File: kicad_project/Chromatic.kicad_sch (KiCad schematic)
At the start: 157 parts

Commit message: arrumadas as bibliotecas
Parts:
- SW_0_R0C0, SW_0_R0C1, SW_0_R0C10, SW_0_R0C11, SW_0_R0C12, SW_0_R0C13, SW_0_R0C14, SW_0_R0C15, SW_0_R0C16, SW_0_R0C2, SW_0_R0C3, SW_0_R0C4, SW_0_R0C5, SW_0_R0C6, SW_0_R0C7, SW_0_R0C8, SW_0_R0C9, SW_1_R1C0, SW_1_R1C1, SW_1_R1C10, SW_1_R1C11, SW_1_R1C12, SW_1_R1C13, SW_1_R1C14, SW_1_R1C15, SW_1_R1C16, SW_1_R1C2, SW_1_R1C3, SW_1_R1C4, SW_1_R1C5, SW_1_R1C6, SW_1_R1C7, SW_1_R1C8, SW_1_R1C9, SW_2_R2C0, SW_2_R2C1, SW_2_R2C10, SW_2_R2C11, SW_2_R2C12, SW_2_R2C13, SW_2_R2C14, SW_2_R2C15, SW_2_R2C16, SW_2_R2C2, SW_2_R2C3, SW_2_R2C4, SW_2_R2C5, SW_2_R2C6, SW_2_R2C7, SW_2_R2C8, SW_2_R2C9, SW_3_R0C0, SW_3_R0C1, SW_3_R0C10, SW_3_R0C11, SW_3_R0C12, SW_3_R0C13, SW_3_R0C14, SW_3_R0C15, SW_3_R0C16, SW_3_R0C2, SW_3_R0C3, SW_3_R0C4, SW_3_R0C5, SW_3_R0C6, SW_3_R0C7, SW_3_R0C8, SW_3_R0C9, SW_4_R1C0, SW_4_R1C1, SW_4_R1C10, SW_4_R1C11, SW_4_R1C12, SW_4_R1C13, SW_4_R1C14, SW_4_R1C15, SW_4_R1C16, SW_4_R1C2, SW_4_R1C3, SW_4_R1C4, SW_4_R1C5, SW_4_R1C6, SW_4_R1C7, SW_4_R1C8, SW_4_R1C9, SW_5_R2C0, SW_5_R2C1, SW_5_R2C10, SW_5_R2C11, SW_5_R2C12, SW_5_R2C13, SW_5_R2C14, SW_5_R2C15, SW_5_R2C16, SW_5_R2C2, SW_5_R2C3, SW_5_R2C4, SW_5_R2C5, SW_5_R2C6, SW_5_R2C7, SW_5_R2C8, SW_5_R2C9: footprint ScottoKeebs_Hotswap:Hotswap_MX_1.00u -> ScottoKeebs_MX:MX_PCB_1.00u

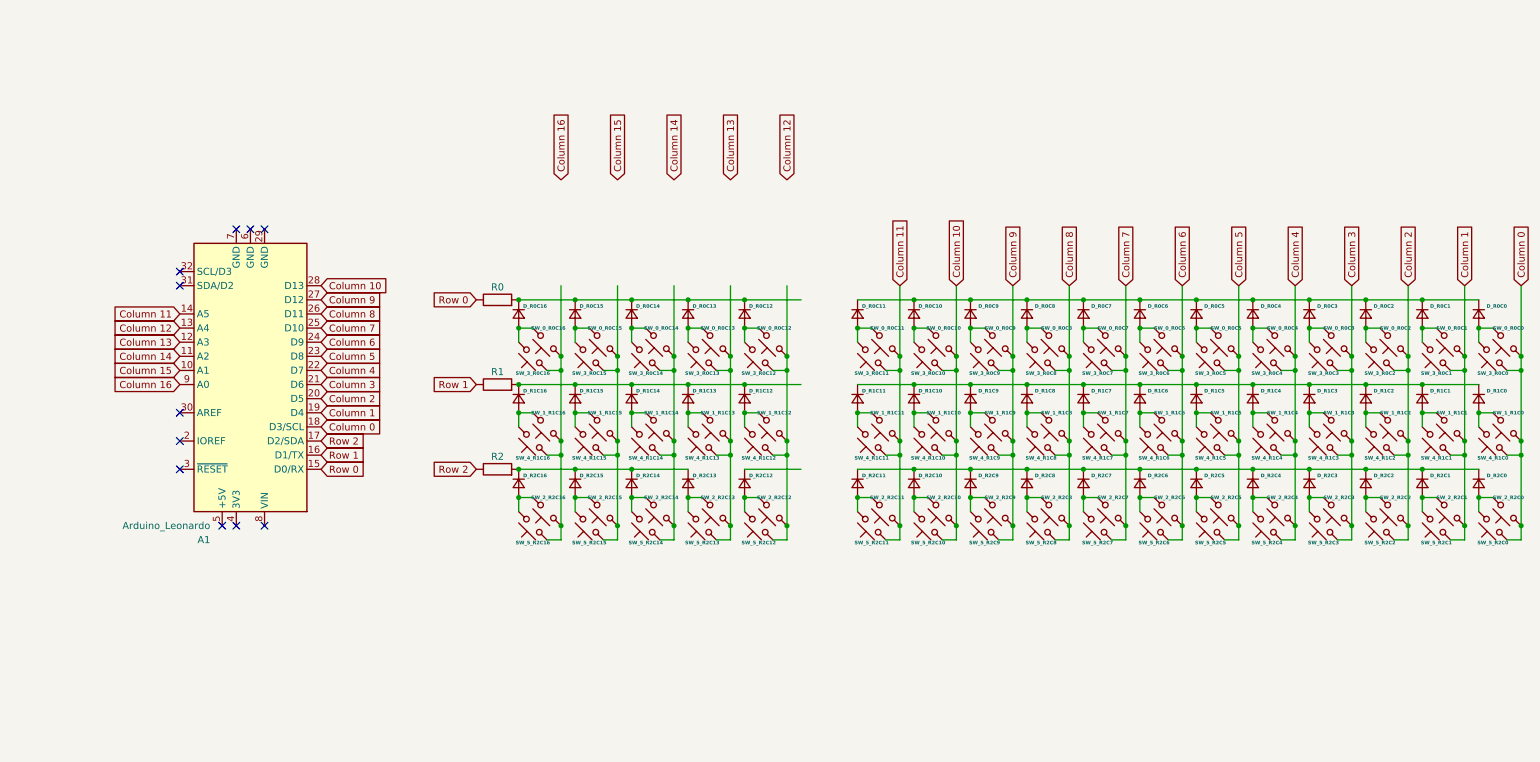
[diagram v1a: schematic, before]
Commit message: commit
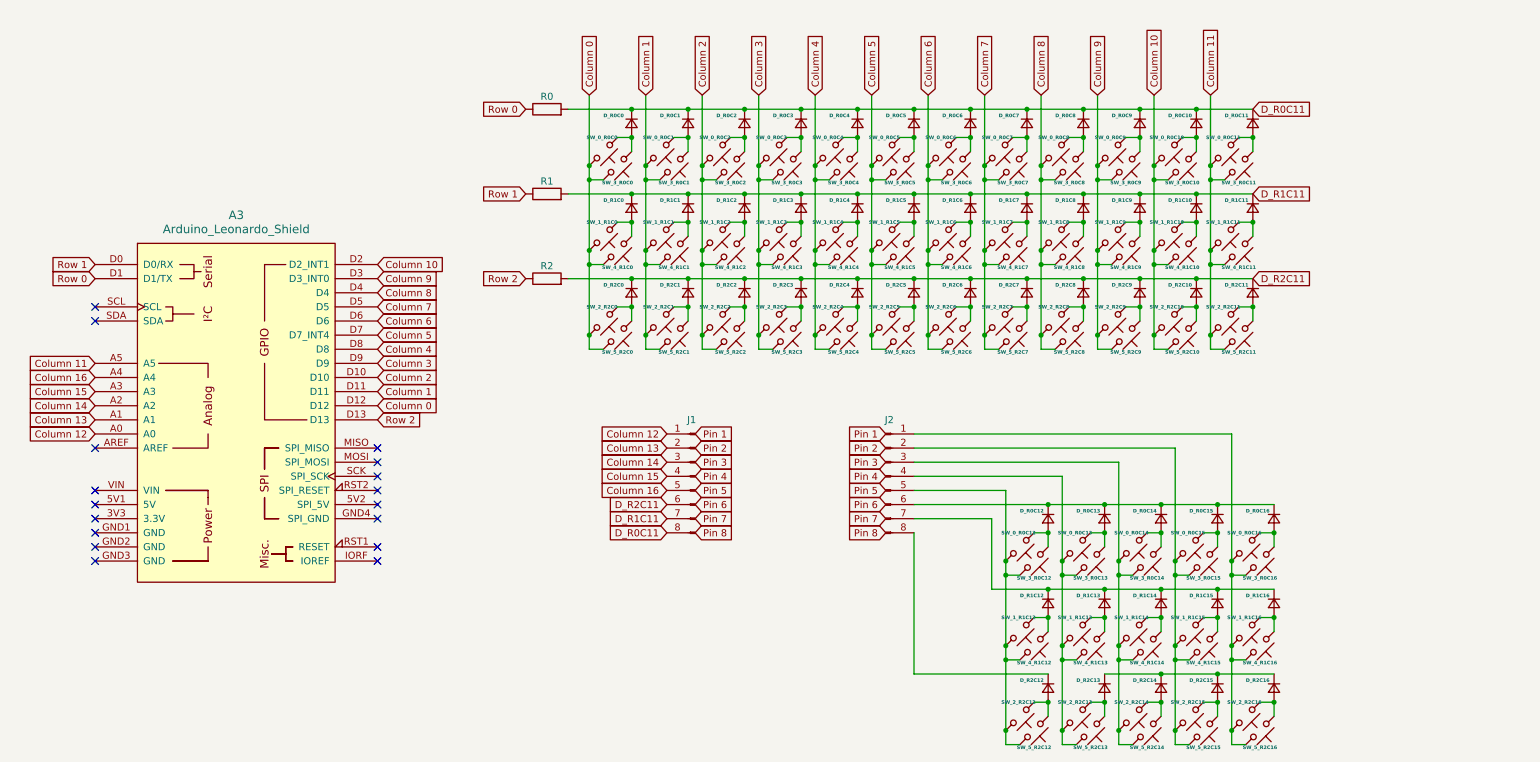
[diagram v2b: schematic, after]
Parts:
- removed A1: Arduino_Leonardo, Module:Arduino_UNO_R3, symbol MCU_Module:Arduino_Leonardo
- added A3: Arduino_Leonardo_Shield, arduino-library:Arduino_Leonardo_Shield, symbol arduino-library:Arduino_Leonardo_Shield
- added J1: J1, Connector_PinHeader_2.54mm:PinHeader_1x08_P2.54mm_Vertical, symbol Connector:Conn_01x08_Pin
- added J2: J2, Connector_PinHeader_2.54mm:PinHeader_1x08_P2.54mm_Vertical, symbol Connector:Conn_01x08_Pin
- SW_0_R0C0, SW_0_R0C1, SW_0_R0C10, SW_0_R0C11, SW_0_R0C12, SW_0_R0C13, SW_0_R0C14, SW_0_R0C15, SW_0_R0C16, SW_0_R0C2, SW_0_R0C3, SW_0_R0C4, SW_0_R0C5, SW_0_R0C6, SW_0_R0C7, SW_0_R0C8, SW_0_R0C9, SW_1_R1C0, SW_1_R1C1, SW_1_R1C10, SW_1_R1C11, SW_1_R1C12, SW_1_R1C13, SW_1_R1C14, SW_1_R1C15, SW_1_R1C16, SW_1_R1C2, SW_1_R1C3, SW_1_R1C4, SW_1_R1C5, SW_1_R1C6, SW_1_R1C7, SW_1_R1C8, SW_1_R1C9, SW_2_R2C0, SW_2_R2C1, SW_2_R2C10, SW_2_R2C11, SW_2_R2C12, SW_2_R2C13, SW_2_R2C14, SW_2_R2C15, SW_2_R2C16, SW_2_R2C2, SW_2_R2C3, SW_2_R2C4, SW_2_R2C5, SW_2_R2C6, SW_2_R2C7, SW_2_R2C8, SW_2_R2C9, SW_3_R0C0, SW_3_R0C1, SW_3_R0C10, SW_3_R0C11, SW_3_R0C12, SW_3_R0C13, SW_3_R0C14, SW_3_R0C15, SW_3_R0C16, SW_3_R0C2, SW_3_R0C3, SW_3_R0C4, SW_3_R0C5, SW_3_R0C6, SW_3_R0C7, SW_3_R0C8, SW_3_R0C9, SW_4_R1C0, SW_4_R1C1, SW_4_R1C10, SW_4_R1C11, SW_4_R1C12, SW_4_R1C13, SW_4_R1C14, SW_4_R1C15, SW_4_R1C16, SW_4_R1C2, SW_4_R1C3, SW_4_R1C4, SW_4_R1C5, SW_4_R1C6, SW_4_R1C7, SW_4_R1C8, SW_4_R1C9, SW_5_R2C0, SW_5_R2C1, SW_5_R2C10, SW_5_R2C11, SW_5_R2C12, SW_5_R2C13, SW_5_R2C14, SW_5_R2C15, SW_5_R2C16, SW_5_R2C2, SW_5_R2C3, SW_5_R2C4, SW_5_R2C5, SW_5_R2C6, SW_5_R2C7, SW_5_R2C8, SW_5_R2C9: footprint ScottoKeebs_MX:MX_PCB_1.00u -> ScottoKeebs_Scotto:MX_Hotswap_1.00u
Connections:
- net Column 0: now also A3.D12
- net Column 1: now also A3.D11
- net Column 10: now also A3.D2 (D2_INT1)
- net Column 11: now also A3.A5
- net Column 12: now also A3.A0, J1.1 (Pin_1)
- net Column 13: now also A3.A1, J1.2 (Pin_2)
- net Column 14: now also A3.A2, J1.3 (Pin_3)
- net Column 15: now also A3.A3, J1.4 (Pin_4)
- net Column 16: now also A3.A4, J1.5 (Pin_5)
- net Column 2: now also A3.D10
- net Column 3: now also A3.D9
- net Column 4: now also A3.D8
- net Column 5: now also A3.D7 (D7_INT4)
- net Column 6: now also A3.D6
- net Column 7: now also A3.D5
- net Column 8: now also A3.D4
- net Column 9: now also A3.D3 (D3_INT0)
- net Row 0: now also A3.D1 (D1/TX)
- net Row 1: now also A3.D0 (D0/RX)
- net Row 2: now also A3.D13
- net D_R2C11: now reaches D_R2C0.1 (K), D_R2C1.1 (K), D_R2C10.1 (K), D_R2C11.1 (K), D_R2C2.1 (K), D_R2C3.1 (K), D_R2C4.1 (K), D_R2C5.1 (K), D_R2C6.1 (K), D_R2C7.1 (K), D_R2C8.1 (K), D_R2C9.1 (K)
- net D_R2C11: now also R2.2, J1.6 (Pin_6)
- net D_R0C11: now reaches D_R0C0.1 (K), D_R0C1.1 (K), D_R0C10.1 (K), D_R0C11.1 (K), D_R0C2.1 (K), D_R0C3.1 (K), D_R0C4.1 (K), D_R0C5.1 (K), D_R0C6.1 (K), D_R0C7.1 (K), D_R0C8.1 (K), D_R0C9.1 (K)
- net D_R0C11: now also R0.2, J1.8 (Pin_8)
- net at D_R1C12.1 (K), D_R1C13.1 (K), D_R1C14.1 (K)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: now also J2.7 (Pin_7); no longer R1.2
- net at SW_0_R0C16.1, SW_1_R1C16.1, SW_2_R2C16.1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: now also J2.1 (Pin_1)
- net D_R1C11: now reaches D_R1C0.1 (K), D_R1C1.1 (K), D_R1C10.1 (K), D_R1C11.1 (K), D_R1C2.1 (K), D_R1C3.1 (K), D_R1C4.1 (K), D_R1C5.1 (K), D_R1C6.1 (K), D_R1C7.1 (K), D_R1C8.1 (K), D_R1C9.1 (K)
- net D_R1C11: now also R1.2, J1.7 (Pin_7)
- net at SW_0_R0C15.1, SW_1_R1C15.1, SW_2_R2C15.1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: now also J2.2 (Pin_2)
- net at D_R0C12.1 (K), D_R0C13.1 (K), D_R0C14.1 (K)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: now also J2.6 (Pin_6); no longer R0.2
- net at SW_0_R0C13.1, SW_1_R1C13.1, SW_2_R2C13.1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: now also J2.4 (Pin_4)
- net at SW_0_R0C14.1, SW_1_R1C14.1, SW_2_R2C14.1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: now also J2.3 (Pin_3)
- net at SW_0_R0C12.1, SW_1_R1C12.1, SW_2_R2C12.1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: now also J2.5 (Pin_5)
- net at D_R2C13.1 (K), D_R2C14.1 (K), D_R2C15.1 (K)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: no longer R2.2
- net at D_R2C12.1 (K): now also J2.8 (Pin_8)
- no-connect marks 11 -> 17
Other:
- moved on the sheet: D_R0C0, D_R0C1, D_R0C10, D_R0C11, D_R0C12, D_R0C13, D_R0C14, D_R0C15, D_R0C16, D_R0C2, D_R0C3, D_R0C4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

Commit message: layout
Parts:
- D_R0C0, D_R0C1, D_R0C10, D_R0C11, D_R0C12, D_R0C13, D_R0C14, D_R0C15, D_R0C16, D_R0C2, D_R0C3, D_R0C4, D_R0C5, D_R0C6, D_R0C7, D_R0C8, D_R0C9, D_R1C0, D_R1C1, D_R1C10, D_R1C11, D_R1C12, D_R1C13, D_R1C14, D_R1C15, D_R1C16, D_R1C2, D_R1C3, D_R1C4, D_R1C5, D_R1C6, D_R1C7, D_R1C8, D_R1C9, D_R2C0, D_R2C1, D_R2C10, D_R2C11, D_R2C12, D_R2C13, D_R2C14, D_R2C15, D_R2C16, D_R2C2, D_R2C3, D_R2C4, D_R2C5, D_R2C6, D_R2C7, D_R2C8, D_R2C9: value ~ -> (none)
- SW_0_R0C0, SW_0_R0C1, SW_0_R0C10, SW_0_R0C11, SW_0_R0C12, SW_0_R0C13, SW_0_R0C14, SW_0_R0C15, SW_0_R0C16, SW_0_R0C2, SW_0_R0C3, SW_0_R0C4, SW_0_R0C5, SW_0_R0C6, SW_0_R0C7, SW_0_R0C8, SW_0_R0C9, SW_1_R1C0, SW_1_R1C1, SW_1_R1C10, SW_1_R1C11, SW_1_R1C12, SW_1_R1C13, SW_1_R1C14, SW_1_R1C15, SW_1_R1C16, SW_1_R1C2, SW_1_R1C3, SW_1_R1C4, SW_1_R1C5, SW_1_R1C6, SW_1_R1C7, SW_1_R1C8, SW_1_R1C9, SW_2_R2C0, SW_2_R2C1, SW_2_R2C10, SW_2_R2C11, SW_2_R2C12, SW_2_R2C13, SW_2_R2C14, SW_2_R2C15, SW_2_R2C16, SW_2_R2C2, SW_2_R2C3, SW_2_R2C4, SW_2_R2C5, SW_2_R2C6, SW_2_R2C7, SW_2_R2C8, SW_2_R2C9, SW_3_R0C0, SW_3_R0C1, SW_3_R0C10, SW_3_R0C11, SW_3_R0C12, SW_3_R0C13, SW_3_R0C14, SW_3_R0C15, SW_3_R0C16, SW_3_R0C2, SW_3_R0C3, SW_3_R0C4, SW_3_R0C5, SW_3_R0C6, SW_3_R0C7, SW_3_R0C8, SW_3_R0C9, SW_4_R1C0, SW_4_R1C1, SW_4_R1C10, SW_4_R1C11, SW_4_R1C12, SW_4_R1C13, SW_4_R1C14, SW_4_R1C15, SW_4_R1C16, SW_4_R1C2, SW_4_R1C3, SW_4_R1C4, SW_4_R1C5, SW_4_R1C6, SW_4_R1C7, SW_4_R1C8, SW_4_R1C9, SW_5_R2C0, SW_5_R2C1, SW_5_R2C10, SW_5_R2C11, SW_5_R2C12, SW_5_R2C13, SW_5_R2C14, SW_5_R2C15, SW_5_R2C16, SW_5_R2C2, SW_5_R2C3, SW_5_R2C4, SW_5_R2C5, SW_5_R2C6, SW_5_R2C7, SW_5_R2C8, SW_5_R2C9: footprint ScottoKeebs_Scotto:MX_Hotswap_1.00u -> ScottoKeebs_Hotswap:Hotswap_MX_1.00u
